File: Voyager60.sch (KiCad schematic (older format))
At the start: 233 parts, among them Q1 2N7002, SW1 5.2x5.2mm, U1 ATmega32U4-MU, U2 PRTR5V0U2X, Y1 16Mhz

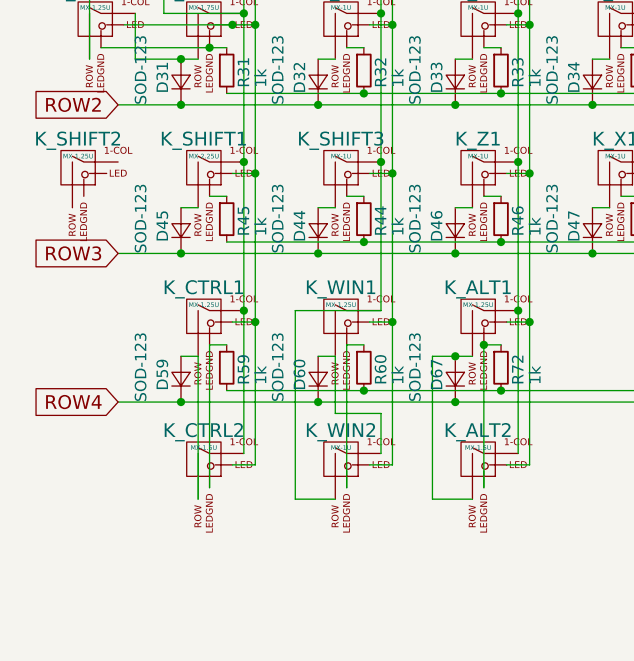
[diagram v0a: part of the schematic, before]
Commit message: Continue routing
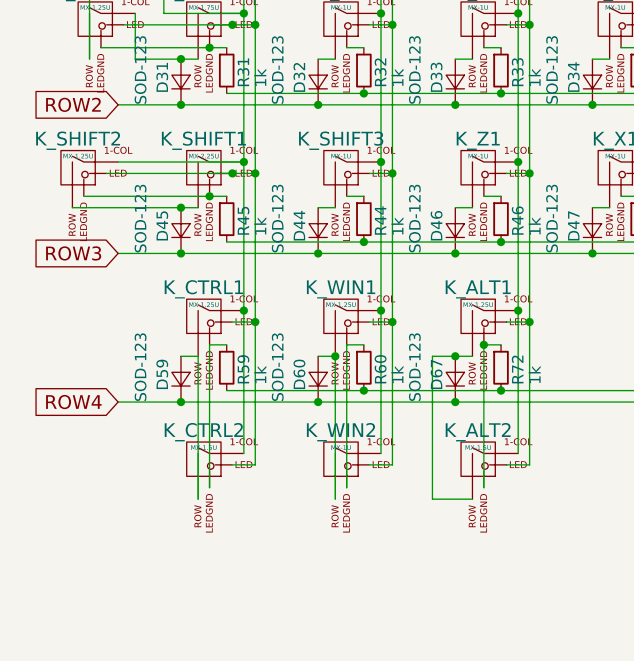
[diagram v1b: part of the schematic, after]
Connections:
- net +5V: now also K_SHIFT2.3 (LED)
- net COL0: now also K_SHIFT2.1 (COL)
- net COL1: now also K_WIN2.1 (COL); no longer K_WIN2.2 (ROW)
- net at D45.2 (A), K_SHIFT1.2 (ROW): now also K_SHIFT2.2 (ROW)
- net at K_SHIFT1.4 (LEDGND), R45.1: now also K_SHIFT2.4 (LEDGND)
- net at D60.2 (A), K_WIN1.2 (ROW): now also K_WIN2.2 (ROW); no longer K_WIN2.1 (COL)
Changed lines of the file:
@@
 	1325 4075 1325 4700
-Wire Wire Line
-	2075 4550 2075 4375
-Wire Wire Line
-	2075 4375 1875 4375
-Wire Wire Line
-	1875 4375 1875 4125
-Wire Wire Line
-	1875 4750 1700 4750
-Wire Wire Line
-	1700 4750 1700 3925
-Wire Wire Line
-	1700 3925 2075 3925
 Wire Wire Line
 	2125 4600 2025 4600
@@
 	9475 3150 9475 3475
 Connection ~ 8475 3475
+Wire Wire Line
+	2075 3925 2075 4550
+Connection ~ 2075 3925
+Wire Wire Line
+	1875 4750 1875 4125
+Connection ~ 1875 4125
+Wire Wire Line
+	1475 3275 925  3275
+Wire Wire Line
+	725  3475 1200 3475
+Connection ~ 1200 3475
+Wire Wire Line
+	1325 3425 775  3425
+Connection ~ 1325 3425
+Wire Wire Line
+	875  3325 1425 3325
+Connection ~ 1425 3325
 $EndSCHEMATC
